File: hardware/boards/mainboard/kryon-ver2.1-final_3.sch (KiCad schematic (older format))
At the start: 3 parts, among them J1 MOLEX_52892-3033MOLEX_52892-3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

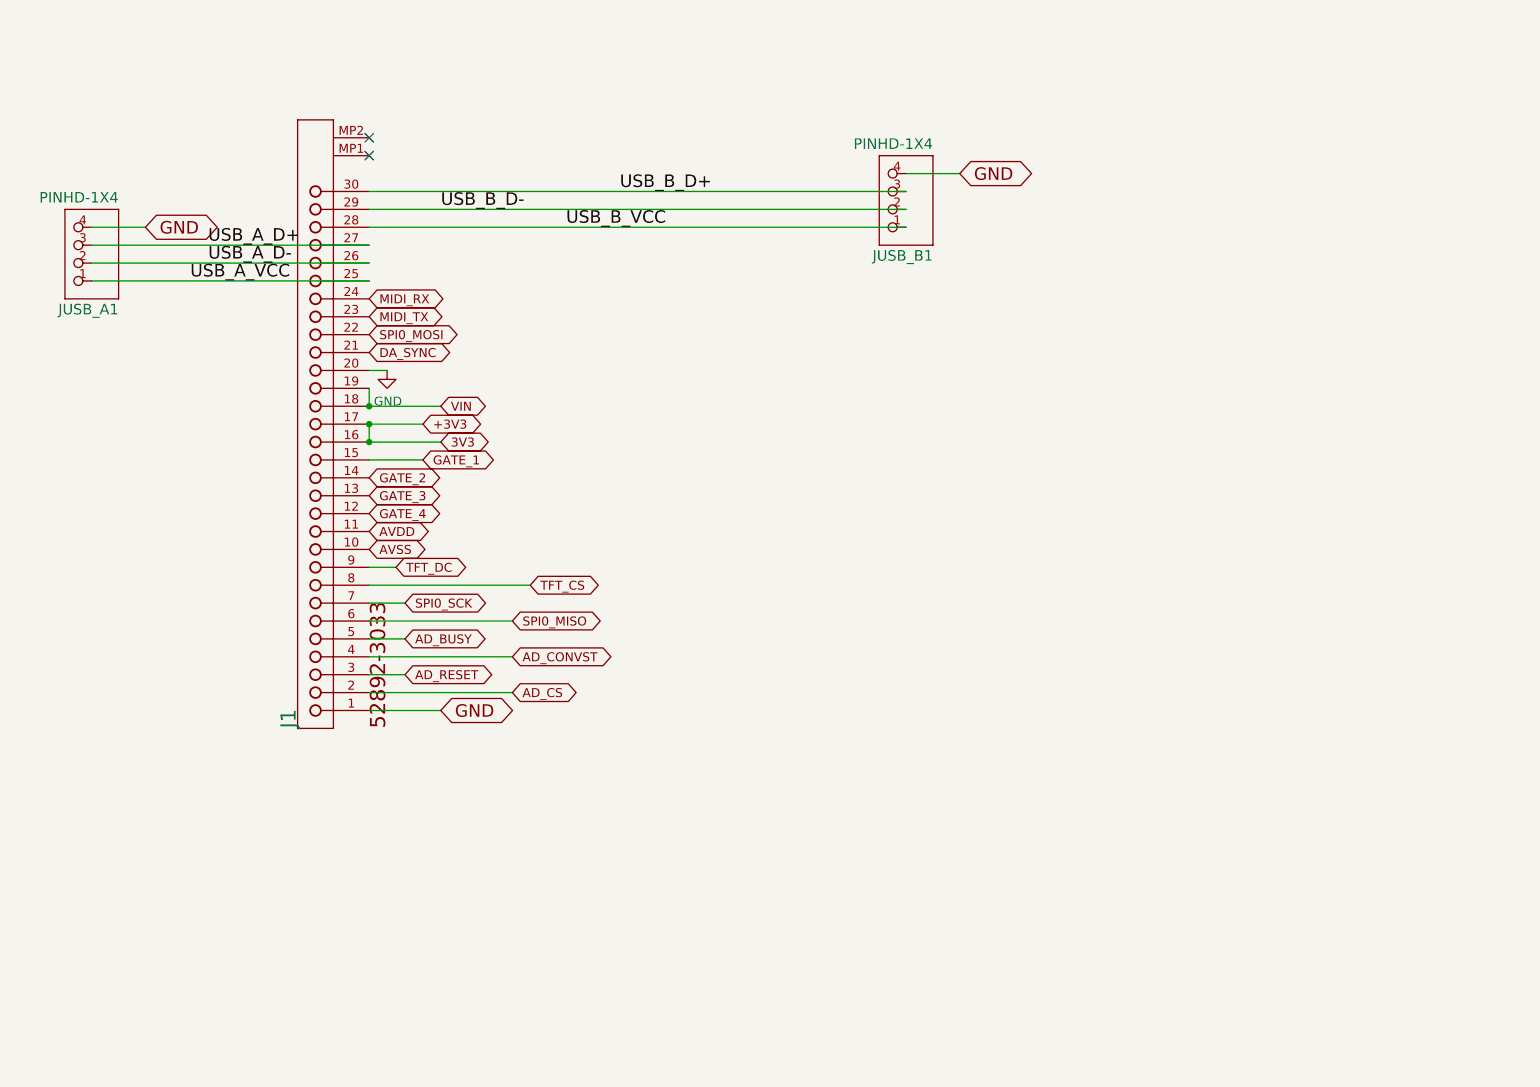
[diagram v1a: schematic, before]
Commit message: mainboard v1.7
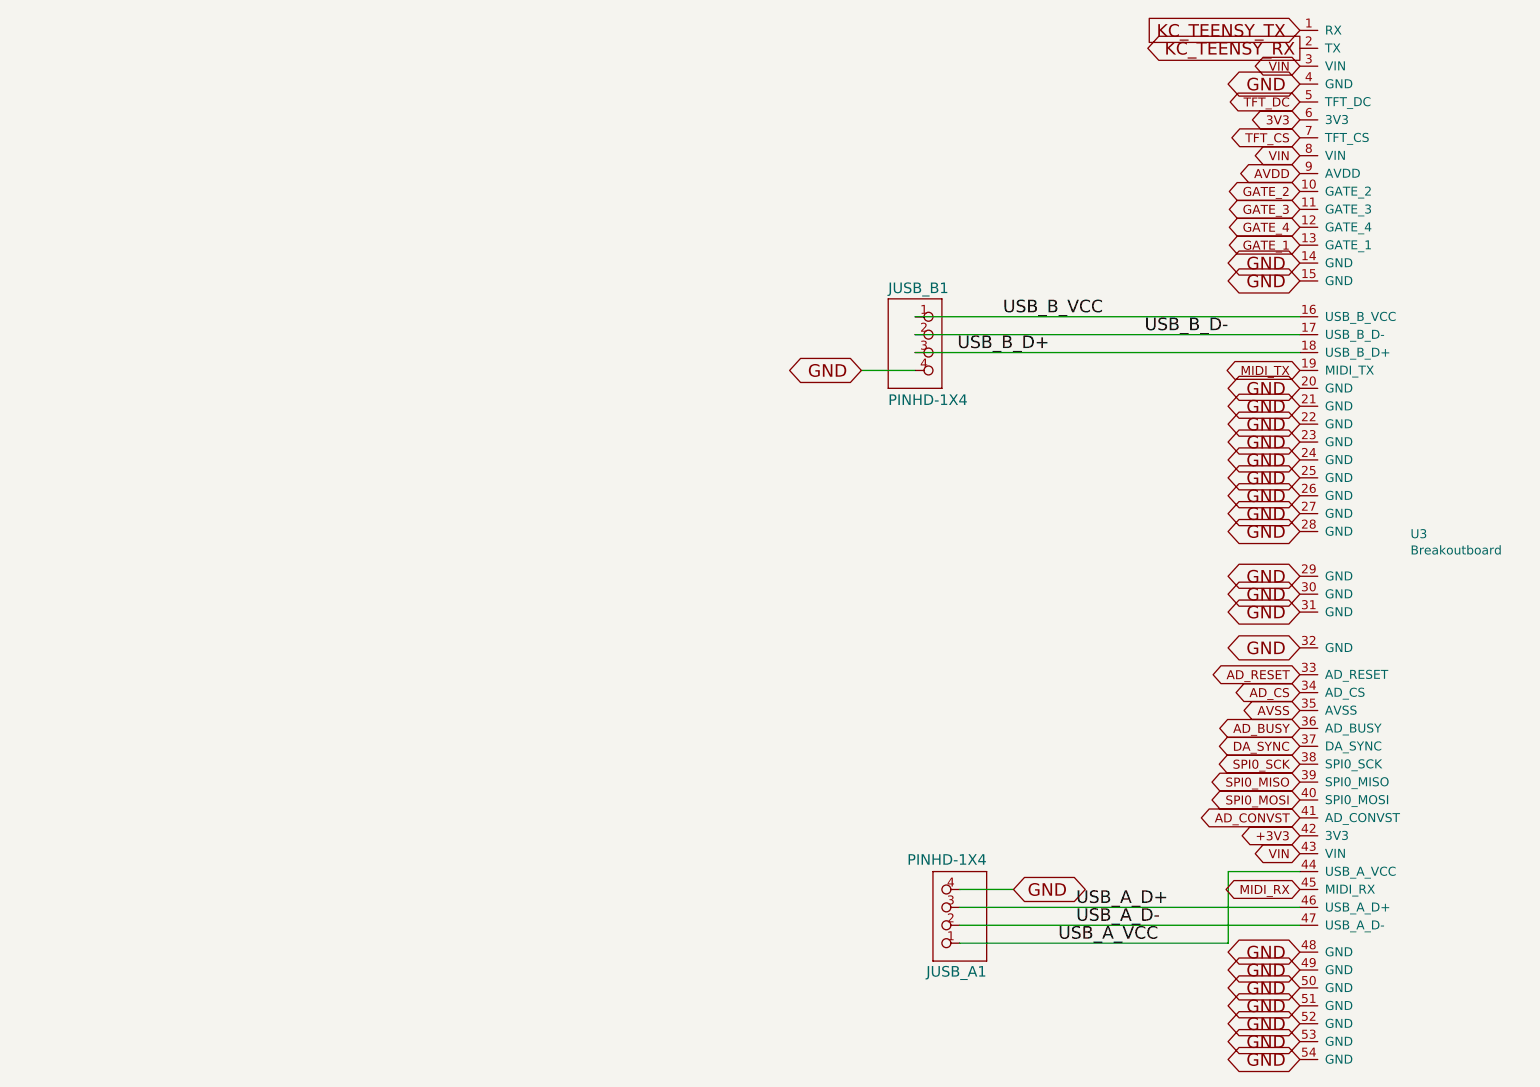
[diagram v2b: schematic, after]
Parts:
- removed J1: MOLEX_52892-3033MOLEX_52892-3033_0_0, Mainboard:MOLEX_52892-3033_0, symbol Mainboard-eagle-import:MOLEX_52892-3033MOLEX_52892-3033_0_0
- added U3: Breakoutboard, topbreakout:Breakoutboard, symbol TopBreakout-eagle-import:Breakoutboard
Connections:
- net +3V3: now also U3.42 (3V3)
- net AD_BUSY: now also U3.36 (AD_BUSY)
- net AD_CONVST: now also U3.41 (AD_CONVST)
- net AD_CS: now also U3.34 (AD_CS)
- net AD_RESET: now also U3.33 (AD_RESET)
- net AVDD: now also U3.9 (AVDD)
- net AVSS: now also U3.35 (AVSS)
- net DA_SYNC: now also U3.37 (DA_SYNC)
- net GATE_1: now also U3.13 (GATE_1)
- net GATE_2: now also U3.10 (GATE_2)
- net GATE_3: now also U3.11 (GATE_3)
- net GATE_4: now also U3.12 (GATE_4)
- net GND: now also U3.14 (GND), U3.15 (GND), U3.20 (GND), U3.21 (GND), U3.22 (GND), U3.23 (GND), U3.24 (GND), U3.25 (GND), U3.26 (GND), U3.27 (GND), U3.28 (GND), U3.29 (GND), U3.30 (GND), U3.31 (GND), U3.32 (GND), U3.4 (GND), U3.48 (GND), U3.49 (GND), U3.50 (GND), U3.51 (GND), U3.52 (GND), U3.53 (GND), U3.54 (GND)
- net MIDI_RX: now also U3.45 (MIDI_RX)
- net MIDI_TX: now also U3.19 (MIDI_TX)
- net SPI0_MISO: now also U3.39 (SPI0_MISO)
- net SPI0_MOSI: now also U3.40 (SPI0_MOSI)
- net SPI0_SCK: now also U3.38 (SPI0_SCK)
- net TFT_CS: now also U3.7 (TFT_CS)
- net TFT_DC: now also U3.5 (TFT_DC)
- net USB_A_D+: now also U3.46 (USB_A_D+)
- net USB_A_D-: now also U3.47 (USB_A_D-)
- net USB_A_VCC: now also U3.44 (USB_A_VCC)
- net USB_B_D+: now also U3.18 (USB_B_D+)
- net USB_B_D-: now also U3.17 (USB_B_D-)
- net USB_B_VCC: now also U3.16 (USB_B_VCC)
- net VIN: now also U3.3 (VIN), U3.43 (VIN), U3.8 (VIN)
- new net 3V3: U3.6 (3V3)
- new net KC_TEENSY_RX: U3.2 (TX)
- new net KC_TEENSY_TX: U3.1 (RX)
- no-connect marks 2 -> 0
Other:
- moved on the sheet: JUSB_A1, JUSB_B1
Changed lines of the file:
@@
-EESchema Schematic File Version 5
+EESchema Schematic File Version 4
 EELAYER 30 0
 EELAYER END
@@
 Comment3 ""
 Comment4 ""
-Comment5 ""
-Comment6 ""
-Comment7 ""
-Comment8 ""
-Comment9 ""
 $EndDescr
+Text GLabel 7250 4700 0    70   BiDi ~ 0
+GND
+Text GLabel 5650 6050 2    70   BiDi ~ 0
+GND
+Text Label 6150 2850 2    70   ~ 0
+USB_B_VCC
+Text Label 6850 2950 2    70   ~ 0
+USB_B_D-
+Text Label 5850 3050 2    70   ~ 0
+USB_B_D+
+Text Label 5900 6350 0    70   ~ 0
+USB_A_VCC
+Text Label 6000 6150 0    70   ~ 0
+USB_A_D+
+Text Label 6000 6250 0    70   ~ 0
+USB_A_D-
+Text GLabel 7250 4950 0    50   BiDi ~ 0
+AD_CS
+Text GLabel 7250 4850 0    50   BiDi ~ 0
+AD_RESET
+Text GLabel 7250 5650 0    50   BiDi ~ 0
+AD_CONVST
+Text GLabel 7250 5150 0    50   BiDi ~ 0
+AD_BUSY
+Text GLabel 7250 5450 0    50   BiDi ~ 0
+SPI0_MISO
+Text GLabel 7250 5350 0    50   BiDi ~ 0
+SPI0_SCK
+Text GLabel 7250 1850 0    50   BiDi ~ 0
+TFT_CS
+Text GLabel 7250 1650 0    50   BiDi ~ 0
+TFT_DC
+Text GLabel 7250 5050 0    50   BiDi ~ 0
+AVSS
+Text GLabel 7250 2050 0    50   BiDi ~ 0
+AVDD
+Text GLabel 7250 2350 0    50   BiDi ~ 0
+GATE_4
+Text GLabel 7250 2250 0    50   BiDi ~ 0
+GATE_3
+Text GLabel 7250 2150 0    50   BiDi ~ 0
+GATE_2
+Text GLabel 7250 2450 0    50   BiDi ~ 0
+GATE_1
+Text GLabel 7250 1750 0    50   BiDi ~ 0
+3V3
+Text GLabel 7250 5750 0    50   BiDi ~ 0
++3V3
+Text GLabel 7250 1950 0    50   BiDi ~ 0
+VIN
 Wire Wire Line
-	2050 5050 2450 5050
-Text GLabel 2450 5050 2    70   BiDi ~ 0
-GND
-Text GLabel 800  2350 2    70   BiDi ~ 0
+	5350 6050 5650 6050
+Wire Wire Line
+	5350 6150 7250 6150
+Wire Wire Line
+	5350 6250 7250 6250
+Wire Wire Line
+	5350 6350 6850 6350
+$Comp
+L Mainboard-eagle-import:PINHD-1X4 JUSB_A1
+U 1 1 A4FDA5DD
+P 5250 6150
+F 0 "JUSB_A1" H 5000 6475 59  0000 L BNN
+F 1 "PINHD-1X4" H 5000 5850 59  0000 L BNN
+F 2 "Mainboard:1X04" H 5250 6150 50  0001 C CNN
+F 3 "" H 5250 6150 50  0001 C CNN
+	1    5250 6150
+	-1   0    0    1
+$EndComp
+Text GLabel 7250 6050 0    50   BiDi ~ 0
+MIDI_RX
+Text GLabel 7250 3150 0    50   BiDi ~ 0
+MIDI_TX
+Text GLabel 7250 5550 0    50   BiDi ~ 0
+SPI0_MOSI
+Text GLabel 7250 5250 0    50   BiDi ~ 0
+DA_SYNC
+$Comp
+L TopBreakout-eagle-import:Breakoutboard U3
+U 1 1 5E131CFF
+P 7900 1150
+F 0 "U3" H 7868 -1764 50  0000 L CNN
+F 1 "Breakoutboard" H 7868 -1855 50  0000 L CNN
+F 2 "topbreakout:Breakoutboard" H 7900 1150 50  0001 C CNN
+F 3 "" H 7900 1150 50  0001 C CNN
+	1    7900 1150
+	1    0    0    -1
+$EndComp
+Text GLabel 4800 3150 0    70   BiDi ~ 0
 GND
 Wire Wire Line
-	5050 2050 5350 2050
-Text Label 3150 2350 0    70   ~ 0
-USB_B_VCC
-Text Label 2450 2250 0    70   ~ 0
-USB_B_D-
-Text Label 3450 2150 0    70   ~ 0
-USB_B_D+
-Text Label 1050 2650 0    70   ~ 0
-USB_A_VCC
-Text Label 1150 2450 0    70   ~ 0
-USB_A_D+
+	7250 2850 5100 2850
 Wire Wire Line
-	2050 3650 2350 3650
+	7250 2950 5100 2950
 Wire Wire Line
-	2050 3550 2450 3550
-Wire Wire Line
-	2050 3450 2350 3450
-Wire Wire Line
-	2050 3350 2450 3350
-Text Label 1150 2550 0    70   ~ 0
-USB_A_D-
-$Comp
-L Mainboard-eagle-import:MOLEX_52892-3033MOLEX_52892-3033_0_0 J1
-U 1 1 F1780596
-P 1450 5150
-F 0 "J1" H 1450 5050 85  0000 L TNN
-F 1 "MOLEX_52892-3033MOLEX_52892-3033_0_0" H 1450 5150 50  0001 C CNN
-F 2 "Mainboard:MOLEX_52892-3033_0" H 1450 5150 50  0001 C CNN
-F 3 "" H 1450 5150 50  0001 C CNN
-	1    1450 5150
-	0    -1   -1   0
-$EndComp
+	7250 3050 5100 3050
 $Comp
 L Mainboard-eagle-import:PINHD-1X4 JUSB_B1
 U 1 1 60AD87F5
-P 4950 2150
-F 0 "JUSB_B1" H 4700 2475 59  0000 L BNN
-F 1 "PINHD-1X4" H 4700 1850 59  0000 L BNN
-F 2 "Mainboard:1X04" H 4950 2150 50  0001 C CNN
-F 3 "" H 4950 2150 50  0001 C CNN
-	1    4950 2150
-	-1   0    0    1
-$EndComp
-Wire Wire Line
-	2050 4950 2850 4950
-Wire Wire Line
-	2050 4850 2250 4850
-Wire Wire Line
-	2050 4750 2850 4750
-Wire Wire Line
-	2050 4650 2250 4650
-Wire Wire Line
-	2050 4550 2850 4550
-Wire Wire Line
-	2050 4450 2250 4450
-Wire Wire Line
-	2050 4250 2200 4250
-Wire Wire Line
-	2050 4350 2950 4350
-Text GLabel 2850 4950 2    50   BiDi ~ 0
-AD_CS
-Text GLabel 2250 4850 2    50   BiDi ~ 0
-AD_RESET
-Text GLabel 2850 4750 2    50   BiDi ~ 0
-AD_CONVST
-Text GLabel 2250 4650 2    50   BiDi ~ 0
-AD_BUSY
-Text GLabel 2850 4550 2    50   BiDi ~ 0
-SPI0_MISO
-Text GLabel 2250 4450 2    50   BiDi ~ 0
-SPI0_SCK
-Text GLabel 2950 4350 2    50   BiDi ~ 0
-TFT_CS
-Text GLabel 2200 4250 2    50   BiDi ~ 0
-TFT_DC
-Text GLabel 2050 4150 2    50   BiDi ~ 0
-AVSS
-Text GLabel 2050 4050 2    50   BiDi ~ 0
-AVDD
-Text GLabel 2050 3950 2    50   BiDi ~ 0
-GATE_4
-Text GLabel 2050 3850 2    50   BiDi ~ 0
-GATE_3
-Text GLabel 2050 3750 2    50   BiDi ~ 0
-GATE_2
-Text GLabel 2350 3650 2    50   BiDi ~ 0
-GATE_1
-Text GLabel 2450 3550 2    50   BiDi ~ 0
-3V3
-Text GLabel 2350 3450 2    50   BiDi ~ 0
-+3V3
-Text GLabel 2450 3350 2    50   BiDi ~ 0
-VIN
-Wire Wire Line
-	500  2350 800  2350
-Wire Wire Line
-	500  2450 2050 2450
-Wire Wire Line
-	500  2550 2050 2550
-Wire Wire Line
-	500  2650 2050 2650
-$Comp
-L Mainboard-eagle-import:PINHD-1X4 JUSB_A1
-U 1 1 A4FDA5DD
-P 400 2450
-F 0 "JUSB_A1" H 150 2775 59  0000 L BNN
-F 1 "PINHD-1X4" H 150 2150 59  0000 L BNN
-F 2 "Mainboard:1X04" H 400 2450 50  0001 C CNN
-F 3 "" H 400 2450 50  0001 C CNN
-	1    400  2450
-	-1   0    0    1
-$EndComp
-Wire Wire Line
-	2050 2150 5050 2150
-Wire Wire Line
-	2050 2250 5050 2250
-Wire Wire Line
-	2050 2350 5050 2350
-Text GLabel 2050 2750 2    50   BiDi ~ 0
-MIDI_RX
-Text GLabel 2050 2850 2    50   BiDi ~ 0
-MIDI_TX
-Text GLabel 2050 2950 2    50   BiDi ~ 0
-SPI0_MOSI
-Text GLabel 2050 3050 2    50   BiDi ~ 0
-DA_SYNC
-$Comp
-L power:GND #PWR0101
-U 1 1 5D91AC47
-P 2150 3150
-F 0 "#PWR0101" H 2150 2900 50  0001 C CNN
-F 1 "GND" H 2155 2977 50  0000 C CNN
-F 2 "" H 2150 3150 50  0001 C CNN
-F 3 "" H 2150 3150 50  0001 C CNN
-	1    2150 3150
+P 5200 3050
+F 0 "JUSB_B1" H 4950 3375 59  0000 L BNN
+F 1 "PINHD-1X4" H 4950 2750 59  0000 L BNN
+F 2 "Mainboard:1X04" H 5200 3050 50  0001 C CNN
+F 3 "" H 5200 3050 50  0001 C CNN
+	1    5200 3050
 	1    0    0    -1
 $EndComp
 Wire Wire Line
-	2150 3150 2050 3150
+	5100 3150 4800 3150
+Text GLabel 7250 5850 0    50   BiDi ~ 0
+VIN
 Wire Wire Line
-	2050 3250 2050 3350
-Connection ~ 2050 3350
+	7250 5950 6850 5950
 Wire Wire Line
-	2050 3550 2050 3450
-Connection ~ 2050 3550
-Connection ~ 2050 3450
-NoConn ~ 2050 1950
-NoConn ~ 2050 1850
-Text GLabel 5350 2050 2    70   BiDi ~ 0
+	6850 5950 6850 6350
+Text GLabel 7250 1450 0    50   BiDi ~ 0
+VIN
+Text GLabel 7250 1350 0    70   Output ~ 0
+KC_TEENSY_RX
+Text GLabel 7250 1250 0    70   Input ~ 0
+KC_TEENSY_TX
+Text GLabel 7250 1550 0    70   BiDi ~ 0
+GND
+Text GLabel 7250 2550 0    70   BiDi ~ 0
+GND
+Text GLabel 7250 2650 0    70   BiDi ~ 0
+GND
+Text GLabel 7250 3250 0    70   BiDi ~ 0
+GND
+Text GLabel 7250 3350 0    70   BiDi ~ 0
+GND
+Text GLabel 7250 3450 0    70   BiDi ~ 0
+GND
+Text GLabel 7250 3550 0    70   BiDi ~ 0
+GND
+Text GLabel 7250 3650 0    70   BiDi ~ 0
+GND
+Text GLabel 7250 3750 0    70   BiDi ~ 0
+GND
+Text GLabel 7250 3850 0    70   BiDi ~ 0
+GND
+Text GLabel 7250 3950 0    70   BiDi ~ 0
+GND
+Text GLabel 7250 4050 0    70   BiDi ~ 0
+GND
+Text GLabel 7250 4300 0    70   BiDi ~ 0
+GND
+Text GLabel 7250 4400 0    70   BiDi ~ 0
+GND
+Text GLabel 7250 4500 0    70   BiDi ~ 0
+GND
+Text GLabel 7250 6400 0    70   BiDi ~ 0
+GND
+Text GLabel 7250 6500 0    70   BiDi ~ 0
+GND
+Text GLabel 7250 6600 0    70   BiDi ~ 0
+GND
+Text GLabel 7250 6700 0    70   BiDi ~ 0
+GND
+Text GLabel 7250 6800 0    70   BiDi ~ 0
+GND
+Text GLabel 7250 6900 0    70   BiDi ~ 0
+GND
+Text GLabel 7250 7000 0    70   BiDi ~ 0
 GND
 $EndSCHEMATC
